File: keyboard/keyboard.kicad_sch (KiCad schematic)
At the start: 91 parts, among them IC1 NRF54L15-QFAA-R, IC2 NPM1300-QEAA-R7, J1 Conn_02x03_Counter_Clockwise

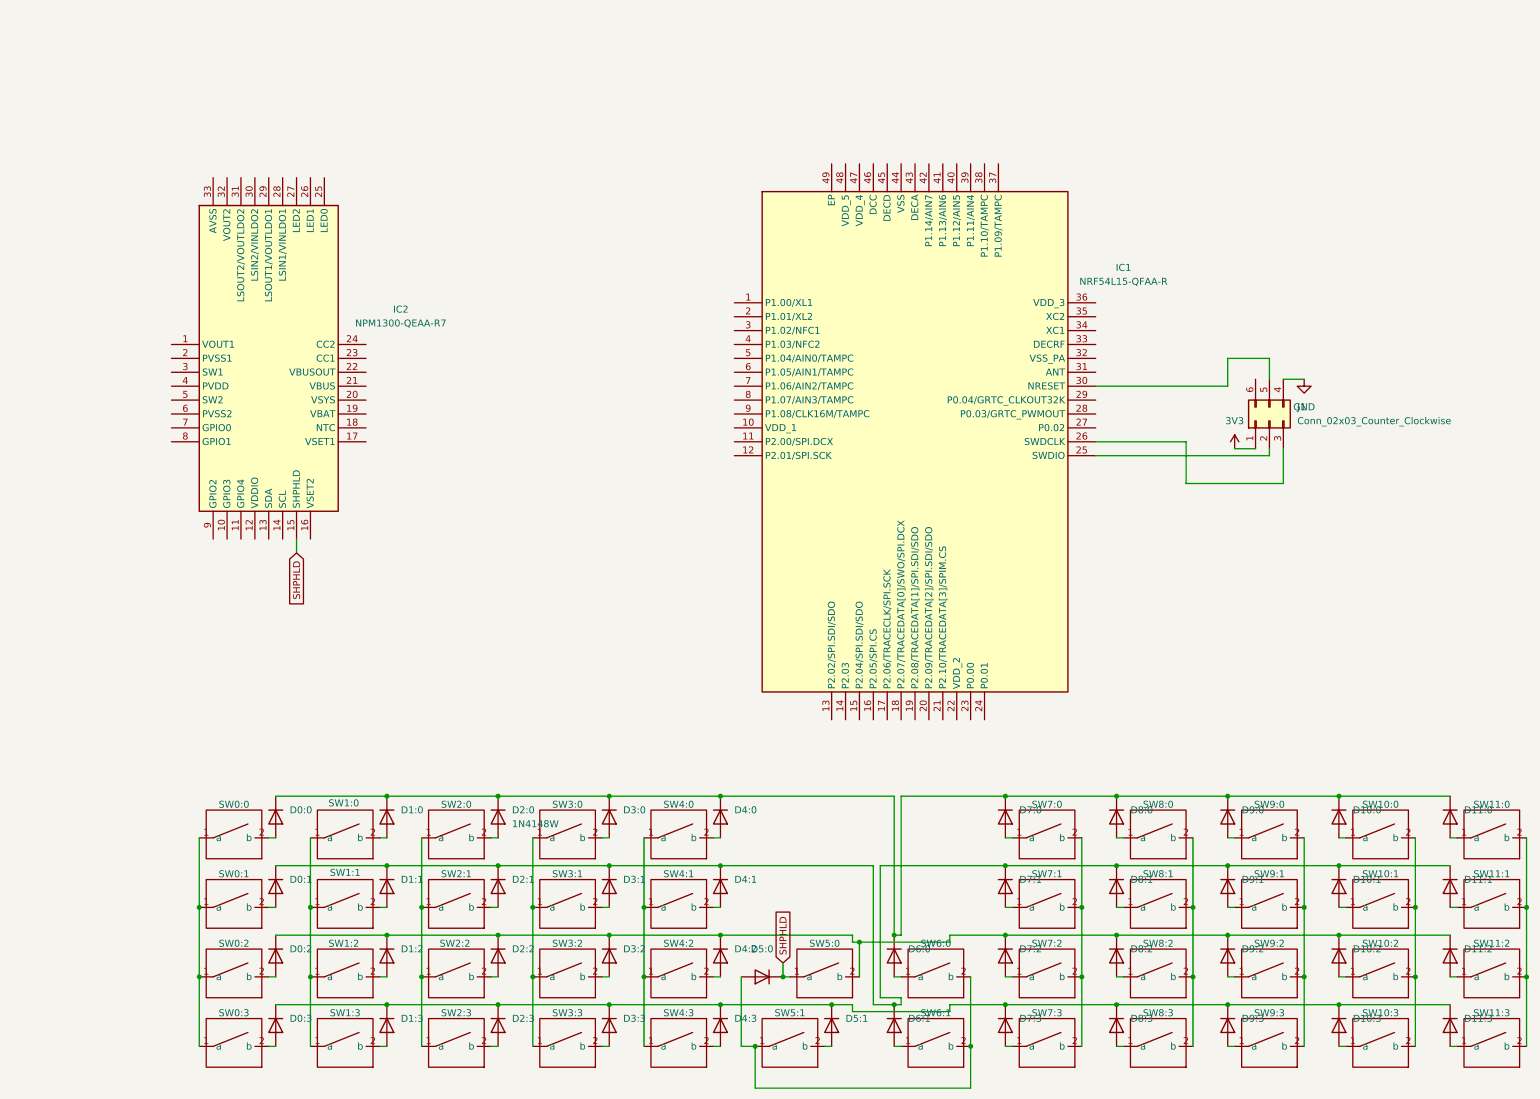
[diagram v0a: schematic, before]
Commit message: ~finished schematic, started layout
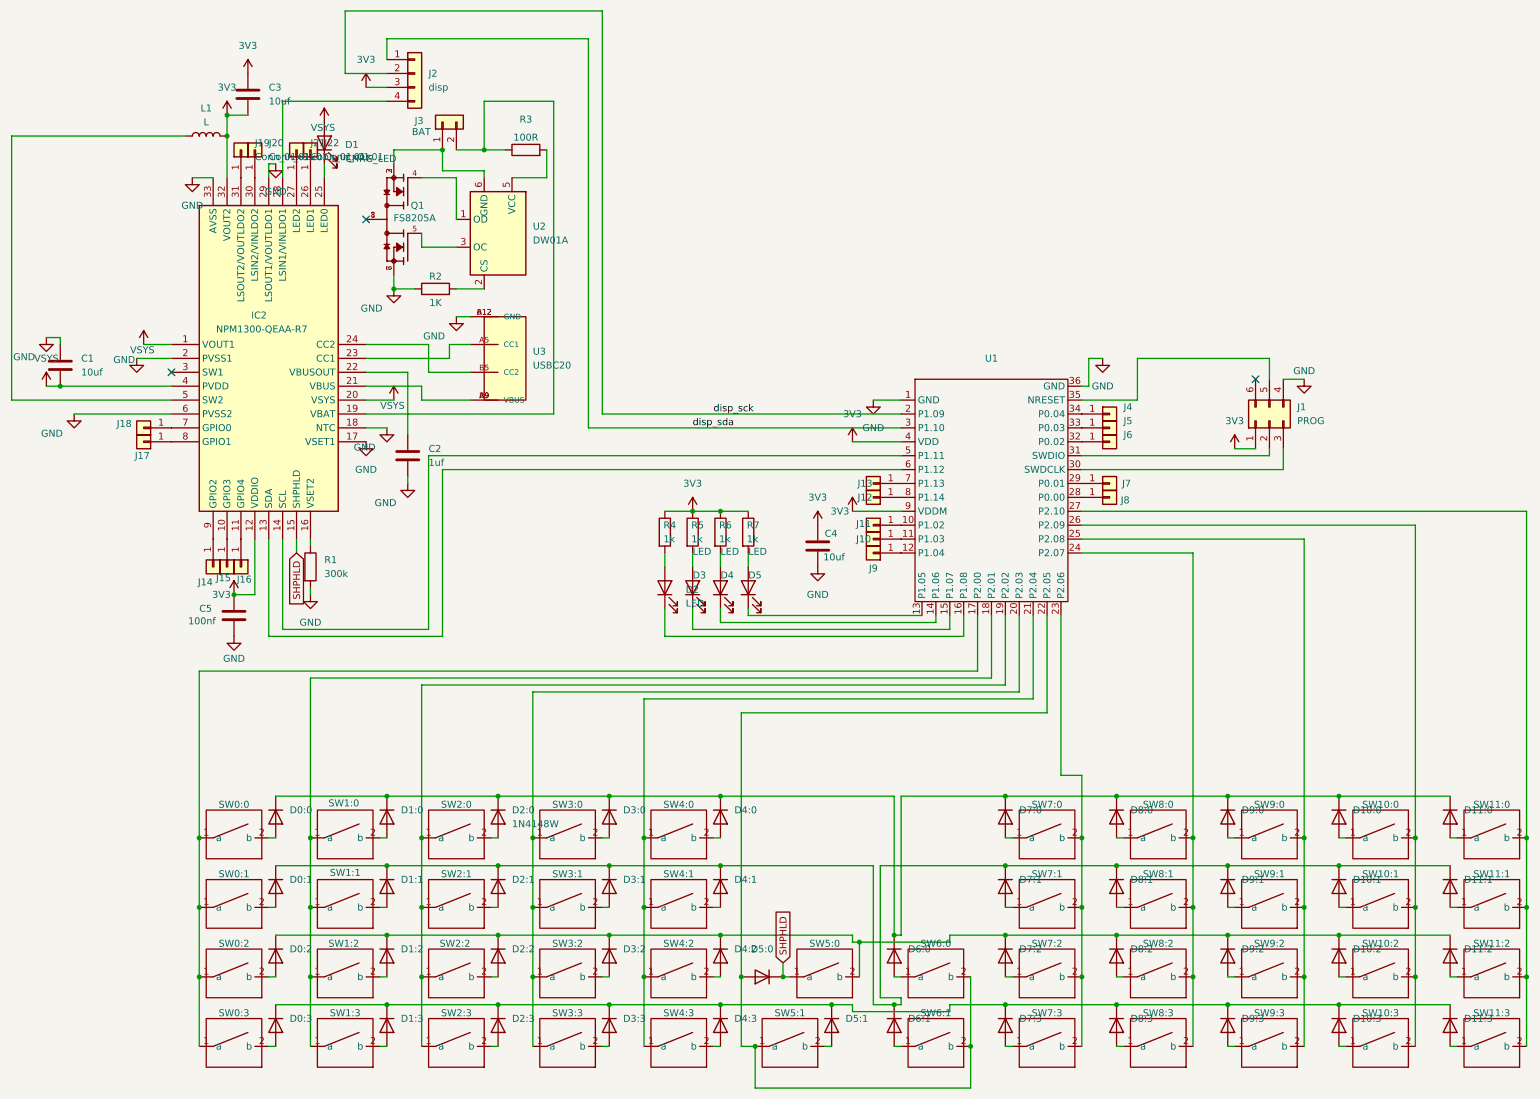
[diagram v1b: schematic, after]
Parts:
- removed IC1: NRF54L15-QFAA-R, QFN40P600X600X95-49N, symbol SamacSys_Parts:NRF54L15-QFAA-R
- added C1, C3, C4: 10uf, Capacitor_SMD:C_0805_2012Metric_Pad1.18x1.45mm_HandSolder, symbol Device:C
- added C2: 1uf, Capacitor_SMD:C_0805_2012Metric_Pad1.18x1.45mm_HandSolder, symbol Device:C
- added C5: 100nf, Capacitor_SMD:C_0805_2012Metric_Pad1.18x1.45mm_HandSolder, symbol Device:C
- added D1: CHRG_LED, LED_SMD:LED_0805_2012Metric_Pad1.15x1.40mm_HandSolder, symbol Device:LED
- added D2, D3, D4, D5: LED, LED_SMD:LED_0805_2012Metric_Pad1.15x1.40mm_HandSolder, symbol Device:LED
- added J10, J11, J12, J13, J14, J15, J16, J17, J18, J19, J20, J21, J22, J4, J5, J6, J7, J8, J9: Conn_01x01, Connector_Wire:SolderWirePad_1x01_SMD_1x2mm, symbol Connector_Generic:Conn_01x01
- added J2: disp, Connector_PinHeader_2.54mm:PinHeader_1x04_P2.54mm_Vertical, symbol Connector_Generic:Conn_01x04
- added J3: BAT, Connector_PinHeader_2.54mm:PinHeader_1x02_P2.54mm_Vertical, symbol Connector_Generic:Conn_01x02
- added L1: L, Inductor_SMD:L_1008_2520Metric_Pad1.43x2.20mm_HandSolder, symbol Device:L
- added Q1: FS8205A, FS8205A:SOP65P640X120-8N, symbol FS8205A:FS8205A
- added R1: 300k, Resistor_SMD:R_0805_2012Metric_Pad1.20x1.40mm_HandSolder, symbol Device:R
- added R2: 1K, Resistor_SMD:R_0805_2012Metric_Pad1.20x1.40mm_HandSolder, symbol Device:R
- added R3: 100R, Resistor_SMD:R_0805_2012Metric_Pad1.20x1.40mm_HandSolder, symbol Device:R
- added R4, R5, R6, R7: 1k, Resistor_SMD:R_0805_2012Metric_Pad1.20x1.40mm_HandSolder, symbol Device:R
- added U1: ~, mylib:nrf54l15_holyiot, symbol mylib:nrf54l15_holyiot
- added U2: DW01A, Package_TO_SOT_SMD:SOT-23-6, symbol Battery_Management:DW01A
- added U3: USBC20, my_usbc:USBC_6PIN, symbol USBC20:USBC20
- IC2: footprint QFN50P500X500X90-33N -> mylib:QFN50P500X500X90-33N
- J1: value Conn_02x03_Counter_Clockwise -> PROG; footprint (none) -> mylib:SWD_PROG_5pin
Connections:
- net 3V3: now also IC2.12 (VDDIO), IC2.32 (VOUT2), C3.1, C3.2, C4.1, C5.1, J2.3 (Pin_3), L1.2, R4.1, R5.1, R6.1, R7.1, U1.4 (VDD), U1.9 (VDDM)
- net GND: now also IC2.17 (VSET1), IC2.18 (NTC), IC2.2 (PVSS1), IC2.29 (LSOUT1/VOUTLDO1), IC2.33 (AVSS), IC2.6 (PVSS2), C1.1, C2.2, C4.2, C5.2, Q1.6, Q1.7, R1.2, R2.1, U1.1 (GND), U1.36 (GND), U3.A12 (GND), U3.B12 (GND)
- net at SW1:0.1 (a), SW1:1.1 (a), SW1:2.1 (a)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: now also U1.18 (P2.01)
- net at SW0:0.1 (a), SW0:1.1 (a), SW0:2.1 (a)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: now also U1.17 (P2.00)
- net at SW4:0.1 (a), SW4:1.1 (a), SW4:2.1 (a)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: now also U1.21 (P2.04)
- net at SW10:0.2 (b), SW10:1.2 (b), SW10:2.2 (b)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: now also U1.26 (P2.09)
- net at SW8:0.2 (b), SW8:1.2 (b), SW8:2.2 (b)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: now also U1.24 (P2.07)
- net at SW2:0.1 (a), SW2:1.1 (a), SW2:2.1 (a)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: now also U1.19 (P2.02)
- net at SW9:0.2 (b), SW9:1.2 (b), SW9:2.2 (b)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: now also U1.25 (P2.08)
- net at D5:0.2 (A), SW5:1.1 (a), SW6:0.2 (b)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: now also U1.22 (P2.05)
- net at SW7:0.2 (b), SW7:1.2 (b), SW7:2.2 (b)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: now also U1.23 (P2.06)
- net at SW11:0.2 (b), SW11:1.2 (b), SW11:2.2 (b)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: now also U1.27 (P2.10)
- net VSYS: now reaches IC2.1 (VOUT1)
- net VSYS: now also IC2.20 (VSYS), IC2.4 (PVDD), C1.2, D1.2 (A)
- net at IC2.10 (GPIO3): now also J15.1 (Pin_1)
- net at IC2.11 (GPIO4): now also J16.1 (Pin_1)
- net at IC2.13 (SDA): now also U1.6 (P1.12)
- net at IC2.14 (SCL): now also U1.5 (P1.11)
- net at IC2.16 (VSET2): now also R1.1
- net at IC2.19 (VBAT): now also J3.2 (Pin_2), R3.1
- net at IC2.21 (VBUS): now also U3.A9 (VBUS), U3.B9 (VBUS)
- net at IC2.22 (VBUSOUT): now also C2.1
- net at IC2.23 (CC1): now also U3.A5 (CC1)
- net at IC2.24 (CC2): now also U3.B5 (CC2)
- net at IC2.25 (LED0): now also D1.1 (K)
- net at IC2.26 (LED1): now also J22.1 (Pin_1)
- net at IC2.27 (LED2): now also J21.1 (Pin_1)
- net at IC2.28 (LSIN1/VINLDO1): now also J2.4 (Pin_4)
- net at IC2.30 (LSIN2/VINLDO2): now also J20.1 (Pin_1)
- net at IC2.31 (LSOUT2/VOUTLDO2): now also J19.1 (Pin_1)
- net at IC2.5 (SW2): now also L1.1
- net at IC2.7 (GPIO0): now also J18.1 (Pin_1)
- net at IC2.8 (GPIO1): now also J17.1 (Pin_1)
- net at IC2.9 (GPIO2): now also J14.1 (Pin_1)
- net at SW3:0.1 (a), SW3:1.1 (a), SW3:2.1 (a)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: now also U1.20 (P2.03)
- net at J1.2 (Pin_2): now also U1.31 (SWDIO)
- net at J1.3 (Pin_3): now also U1.30 (SWDCLK)
- net at J1.5 (Pin_5): now also U1.35 (NRESET)
- new net: D3.1 (K), U1.15 (P1.07)
- new net: D3.2 (A), R5.2
- new net: J3.1 (Pin_1), Q1.2, Q1.3, U2.6 (GND)
- new net: J8.1 (Pin_1), U1.28 (P0.00)
- new net: D2.2 (A), R4.2
- new net: D2.1 (K), U1.16 (P1.08)
- new net: J13.1 (Pin_1), U1.7 (P1.13)
- new net: J6.1 (Pin_1), U1.32 (P0.02)
- new net: J11.1 (Pin_1), U1.10 (P1.02)
- new net: J10.1 (Pin_1), U1.11 (P1.03)
- new net: J9.1 (Pin_1), U1.12 (P1.04)
- new net: D5.1 (K), U1.13 (P1.05)
- new net: D4.1 (K), U1.14 (P1.06)
- new net: J7.1 (Pin_1), U1.29 (P0.01)
- new net: J5.1 (Pin_1), U1.33 (P0.03)
- new net: J4.1 (Pin_1), U1.34 (P0.04)
- new net: J12.1 (Pin_1), U1.8 (P1.14)
- new net: R3.2, U2.5 (VCC)
- new net: D4.2 (A), R6.2
- new net: D5.2 (A), R7.2
- new net: R2.2, U2.2 (CS)
- new net: Q1.1, Q1.8
- new net: Q1.4, U2.1 (OD)
- new net: Q1.5, U2.3 (OC)
- new net disp_sck: J2.2 (Pin_2), U1.2 (P1.09)
- new net disp_sda: J2.1 (Pin_1), U1.3 (P1.10)
- no-connect marks 0 -> 3
